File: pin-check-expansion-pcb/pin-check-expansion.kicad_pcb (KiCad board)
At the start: 2 copper layers, 18 parts, among them SW1 MX-NoLED, SW2 MX-NoLED, U1 MCP23008-xP

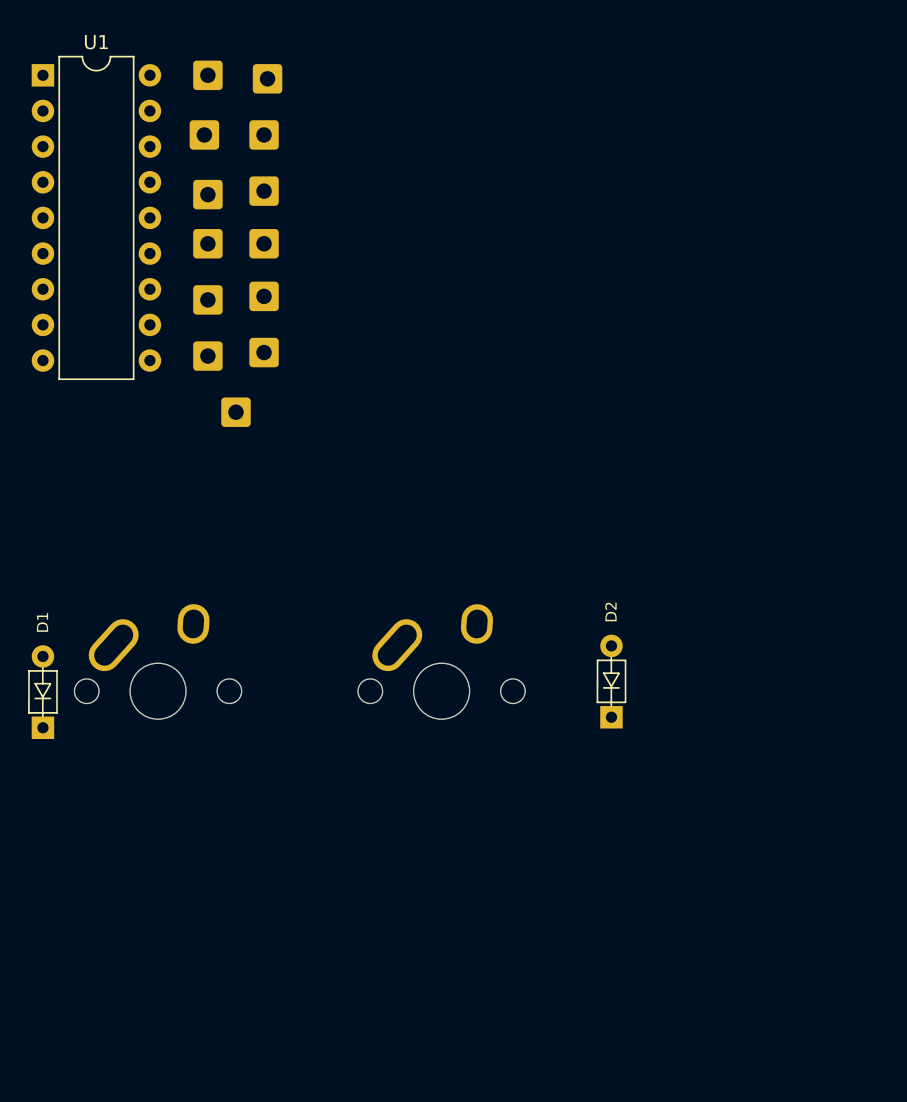
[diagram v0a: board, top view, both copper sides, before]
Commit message: pre-breakout board expirement commit
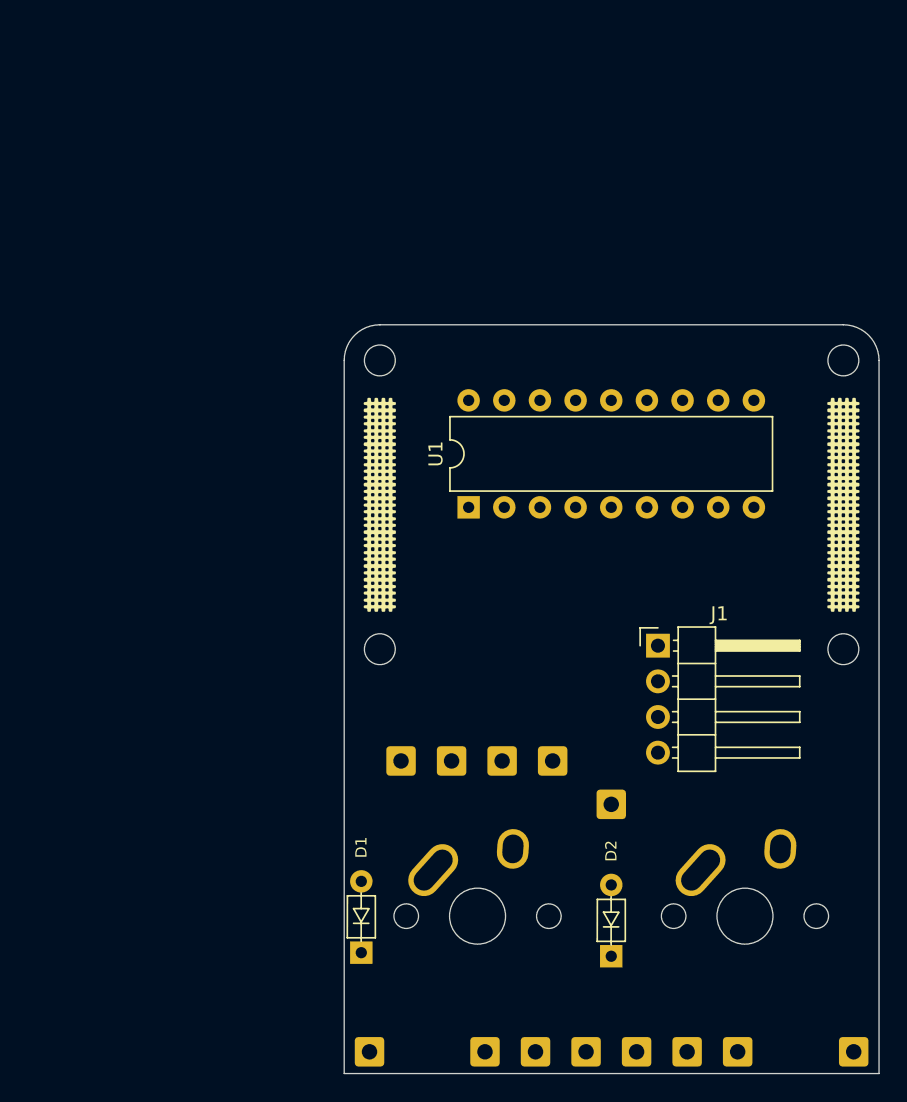
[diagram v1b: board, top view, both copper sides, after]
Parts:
- removed the H1 at (150.8, 63.2)
- removed the H2 at (150.5, 67.2)
- removed the H4 at (150.5, 75.0)
- removed the H7 at (146.5, 63.0)
- added G***: LOGO, pin-check-expansion.pretty:pin-check-pattern, F.Cu at (191.8, 93.6)
- added G***: LOGO, pin-check-expansion.pretty:pin-check-pattern, F.Cu at (158.8, 93.6)
- added H10: MountingHole_Pad, Connector_Wire:SolderWire-0.5sqmm_1x01_D0.9mm_OD2.1mm, B.Cu at (160.3, 111.8)
- added H11: MountingHole_Pad, Connector_Wire:SolderWire-0.5sqmm_1x01_D0.9mm_OD2.1mm, B.Cu at (163.9, 111.8)
- added H12: MountingHole_Pad, Connector_Wire:SolderWire-0.5sqmm_1x01_D0.9mm_OD2.1mm, B.Cu at (167.5, 111.8)
- added H13: MountingHole_Pad, Connector_Wire:SolderWire-0.5sqmm_1x01_D0.9mm_OD2.1mm, B.Cu at (171.1, 111.8)
- added H14: MountingHole_Pad, MountingHole:MountingHole_2.2mm_M2, F.Cu at (158.8, 83.3)
- added H15: MountingHole_Pad, MountingHole:MountingHole_2.2mm_M2, F.Cu at (191.8, 83.3)
- added H16: MountingHole_Pad, MountingHole:MountingHole_2.2mm_M2, F.Cu at (158.8, 103.9)
- added H17: MountingHole_Pad, MountingHole:MountingHole_2.2mm_M2, F.Cu at (191.8, 103.9)
- added J1: Conn_01x04, Connector_PinHeader_2.54mm:PinHeader_1x04_P2.54mm_Horizontal, F.Cu at (178.6, 103.6)
- D1, D2: value D -> 1N4148
- moved H4 75.6 mm to (184.2, 132.6)
- moved H3 74.3 mm to (192.5, 132.6)
- moved H5 70.0 mm to (180.6, 132.6)
- moved H6 65.2 mm to (177.0, 132.6)
- moved H7 60.0 mm to (173.4, 132.6)
- moved H8 54.8 mm to (169.8, 132.6)
- moved H1 54.3 mm to (158.0, 132.6)
- moved H9 48.9 mm to (166.2, 132.6)
- moved U1 43.2 mm to (165.1, 93.8), turned to 90 degrees
- moved H2 40.6 mm to (175.2, 114.9)
- moved SW1 27.8 mm to (165.7, 122.9)
- moved D1 27.8 mm to (157.4, 126.8)
- moved SW2 26.9 mm to (184.8, 122.9)
- moved D2 17.0 mm to (175.2, 127.0)
- renumbered H5 to H1, H6 to H2, H8 to H4, H9 to H5, H10 to H6, H11 to H7, H12 to H8, H13 to H9
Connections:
- H3 pad 1: /SDA -> /ColF
- U1 pad 18: /VCC -> +5V
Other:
- board outline added: 38.1 x 53.3 mm
- board text added: "GND"
- board text added: "I2C"
- board text added: "SCL"
- board text added: "SDA"
- board text added: "VCC"
